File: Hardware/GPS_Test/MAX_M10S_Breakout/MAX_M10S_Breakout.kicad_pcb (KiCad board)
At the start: 2 copper layers, 14 parts, among them J1 U.FL-R-SMT(01), J2 Conn_01x10, U1 MAX-M10S

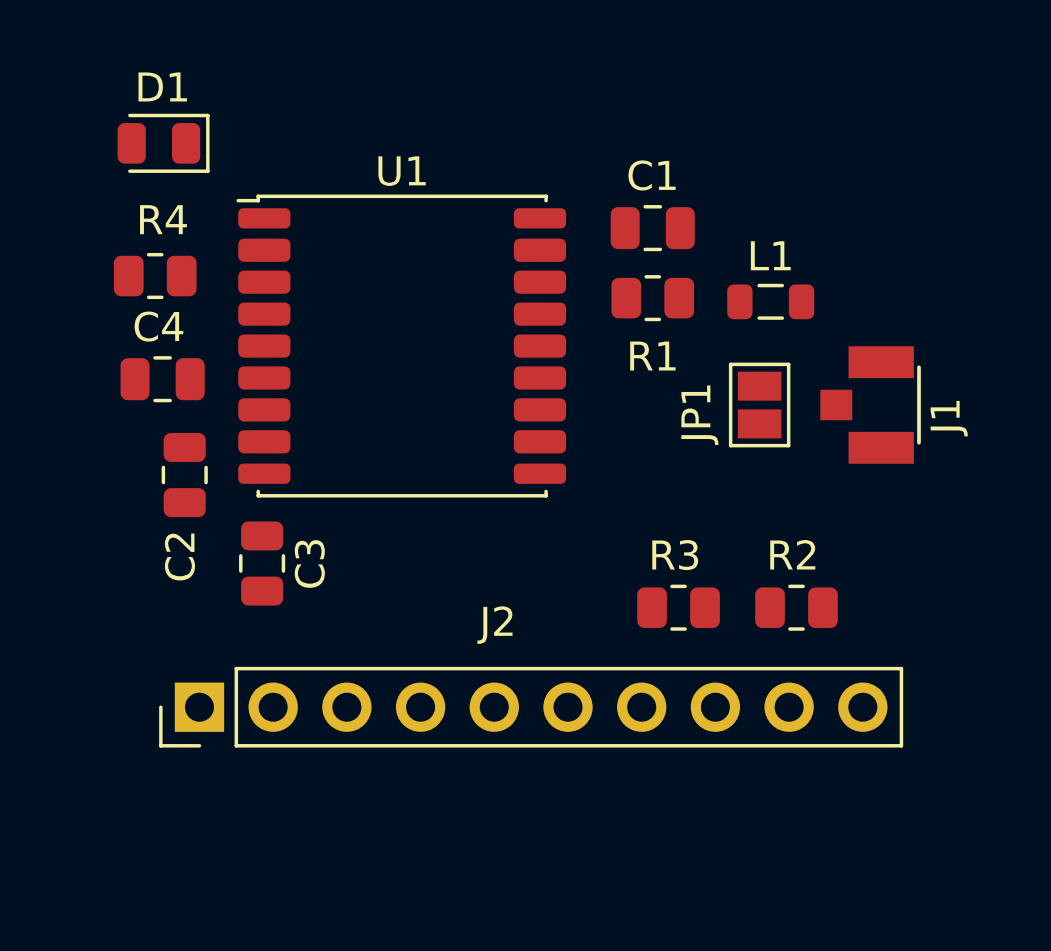
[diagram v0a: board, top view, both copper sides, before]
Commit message: Weiter Max M10S
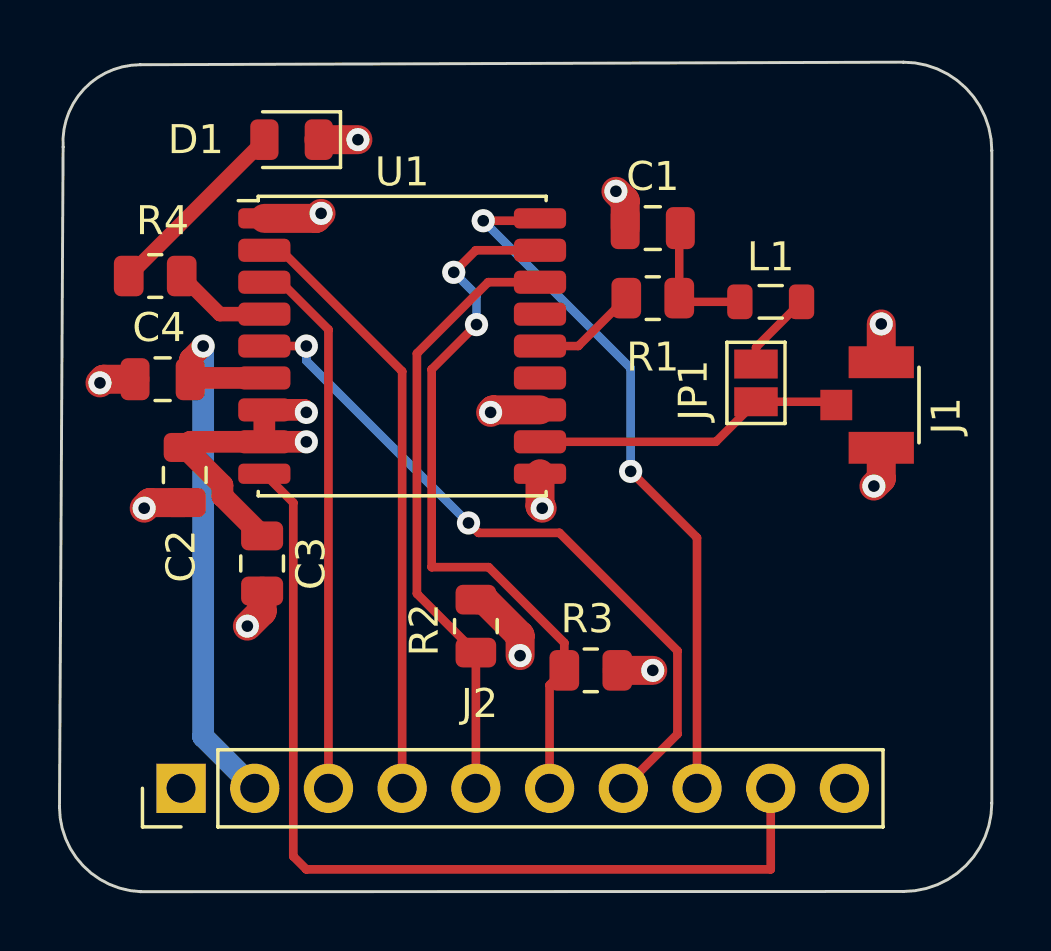
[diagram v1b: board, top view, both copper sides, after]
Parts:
- moved R2 11.1 mm to (94.0, 63.0), turned to -90 degrees
- moved D1 4.57 mm to (87.6, 46.2)
- moved R3 3.72 mm to (97.9, 64.5)
- moved J2 2.87 mm to (83.8, 68.6)
- moved JP1 0.77 mm to (103.6, 54.6)
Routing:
- net ~{RESET}: track 0.00 -> 33.0 mm
- net SCL: track 0.00 -> 25.3 mm, vias 0 -> 2
- net ~{SAFE}: track 0.00 -> 24.6 mm, vias 0 -> 2
- net INT: track 0.00 -> 24.4 mm, vias 0 -> 2
- net SDA: track 0.00 -> 21.1 mm
- net TX: track 0.00 -> 20.8 mm
- net +BATT: track 0.00 -> 19.9 mm, vias 0 -> 1
- net RX: track 0.00 -> 18.7 mm
- net +3.3V: track 0.00 -> 15.0 mm, vias 0 -> 4
- net GND: track 0.00 -> 14.6 mm, vias 0 -> 10
- net Net-(J1-SIG): track 0.00 -> 10.8 mm
- net Net-(D1-A): track 0.00 -> 6.64 mm
- net Net-(C1-Pad1): track 0.00 -> 4.57 mm
- net Net-(U1-VCC_RF): track 0.00 -> 3.66 mm
- net PPS: track 0.00 -> 3.39 mm
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- added copper zone on In2.Cu, net +3.3V
- added copper zone on In1.Cu, net GND
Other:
- board outline added: 32.1 x 28.6 mm
- copper layers 2 -> 4
